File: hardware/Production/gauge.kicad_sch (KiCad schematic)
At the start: 68 parts, among them J105 Cell 2 NTC wires, J106 Cell 3 NTC wires, J108 PACK- power wire, J109 CELL1 sense wire, J110 CELL2 sense wire, J111 CELL3 sense wire, J112 PACK+ power wire, J113 LOAD PACK_P, J114 LOAD GND, J115 1N Kelvin wire, J116 4P Kelvin wire, Q101 BSC007N04LS6, Q102 BSC007N04LS6, Q103 AO3400A, Q104 AO3400A, U101 BQ40Z50RSMR-R2, U102 BQ294700DSGR

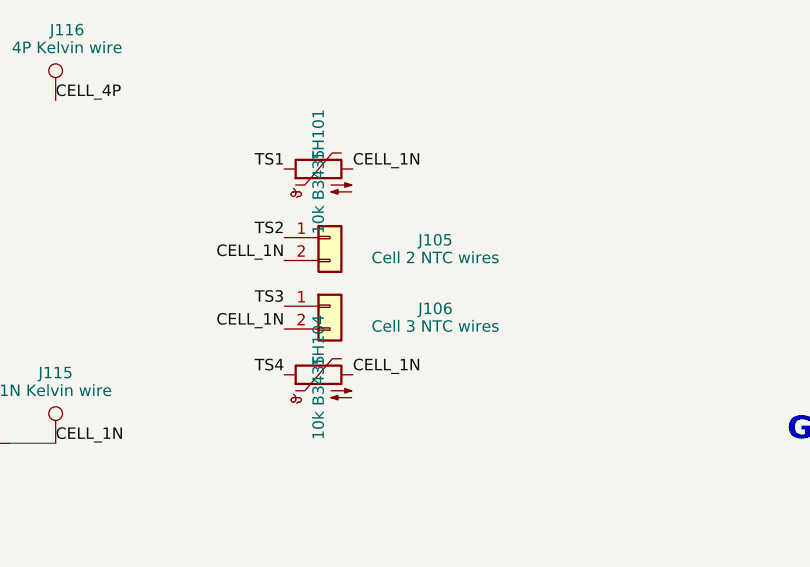
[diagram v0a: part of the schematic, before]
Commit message: Board Layout Done Going to review
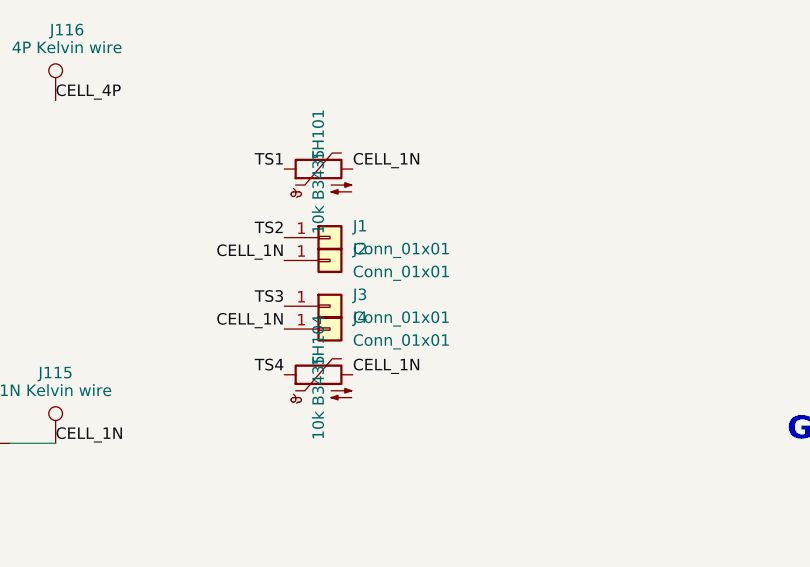
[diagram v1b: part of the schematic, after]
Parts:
- removed J105: Cell 2 NTC wires, Connector_Wire:SolderWire-0.15sqmm_1x02_P4mm_D0.5mm_OD1.5mm, symbol Connector_Generic:Conn_01x02
- removed J106: Cell 3 NTC wires, Connector_Wire:SolderWire-0.15sqmm_1x02_P4mm_D0.5mm_OD1.5mm, symbol Connector_Generic:Conn_01x02
- added J1, J2, J3, J4: Conn_01x01, MonolithDev:SolderWire-28AWG_PTFE_1x01_D0.8mm_Pad1.5x1.4mm, symbol Connector_Generic:Conn_01x01
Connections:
- net CELL_1N: now also J2.1 (Pin_1), J4.1 (Pin_1)
- net TS2: now also J1.1 (Pin_1)
- net TS3: now also J3.1 (Pin_1)

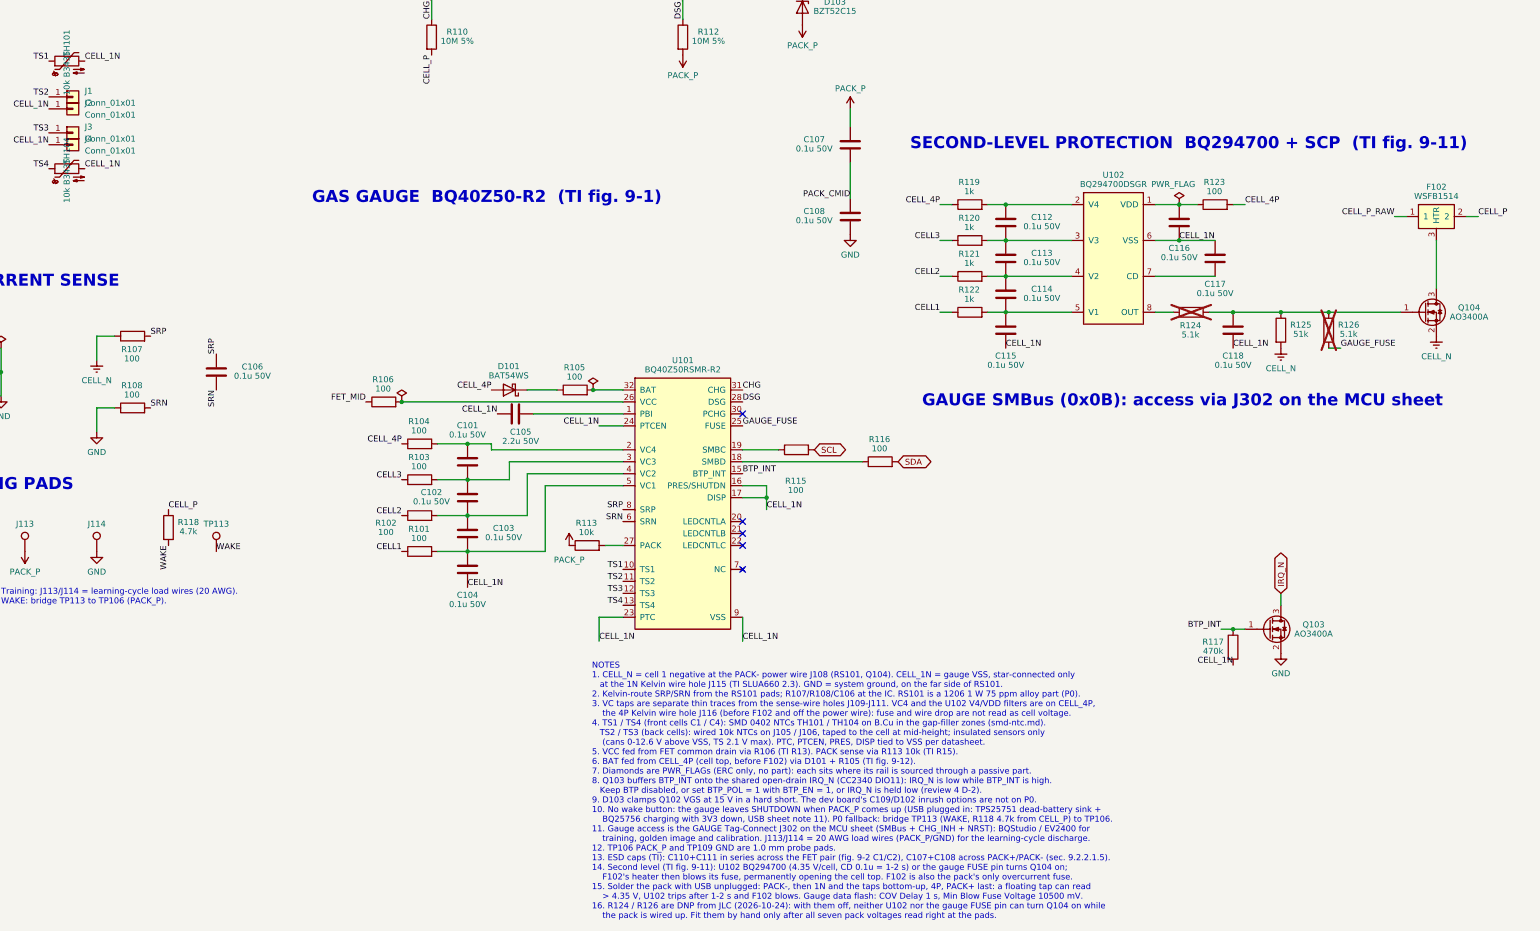
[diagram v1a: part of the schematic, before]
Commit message: Routing fixes done, ready for final review
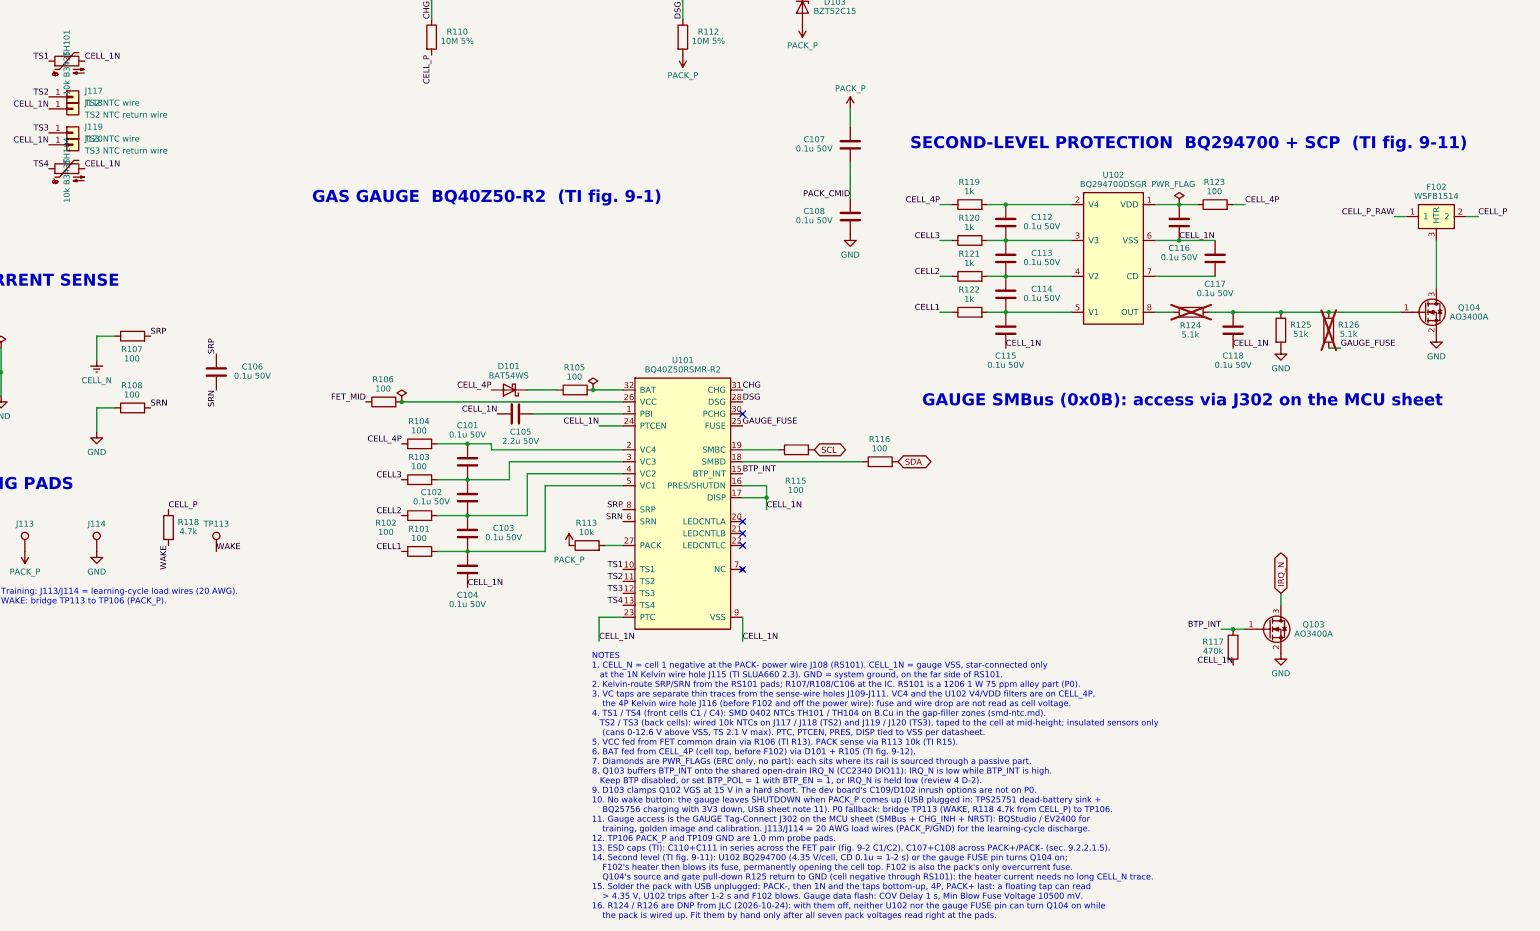
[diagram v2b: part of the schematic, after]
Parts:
- J117: renamed from J1; value Conn_01x01 -> TS2 NTC wire; now left out of the parts list
- J118: renamed from J2; value Conn_01x01 -> TS2 NTC return wire; now left out of the parts list
- J119: renamed from J3; value Conn_01x01 -> TS3 NTC wire; now left out of the parts list
- J120: renamed from J4; value Conn_01x01 -> TS3 NTC return wire; now left out of the parts list
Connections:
- net CELL_N: no longer Q104.2 (S), R125.2
- net GND: now also Q104.2 (S), R125.2
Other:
- note added: "NOTES 1. CELL_N = cell 1 negative at the PACK- power wire J108 (RS101). CELL_1N = gauge VSS, star-connected only at the 1N Kelvin wire hole J115 (TI SLUA660 2.3). GND = system ground, on the far side of RS101. 2. Kelvin-route SRP/SRN from the RS101 pads; R107/R108/C106 at the IC. RS101 is a 1206 1 W 75 ppm alloy part (P0). 3. VC taps are separate thin traces from the sense-wire holes J109-J111. V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"
- note removed: "NOTES 1. CELL_N = cell 1 negative at the PACK- power wire J108 (RS101, Q104). CELL_1N = gauge VSS, star-connected only at the 1N Kelvin wire hole J115 (TI SLUA660 2.3). GND = system ground, on the far side of RS101. 2. Kelvin-route SRP/SRN from the RS101 pads; R107/R108/C106 at the IC. RS101 is a 1206 1 W 75 ppm alloy part (P0). 3. VC taps are separate thin traces from the sense-wire holes J109-J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"
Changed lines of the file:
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@@
 		)
 	)
-	(text "NOTES\n1. CELL_N = cell 1 negative at the PACK- power wire J108 (RS101, Q104). CELL_1N = gauge VSS, star-connected only\n   at the 1N Kelvin wire hole J115 (TI SLUA660 2.3). GND = system ground, on the far side of RS101.\n2. Kelvin-route SRP/SRN from the RS101 pads; R107/R108/C106 at the IC. RS101 is a 1206 1 W 75 ppm alloy part (P0).\n3. VC taps are separate thin traces from the sense-wire holes J109-J111. VC4 and the U102 V4/VDD filters are on CELL_4P,\n    the 4P Kelvin wire hole J116 (before F102 and off the power wire): fuse and wire drop are not read as cell voltage.\n4. TS1 / TS4 (front cells C1 / C4): SMD 0402 NTCs TH101 / TH104 on B.Cu in the gap-filler zones (smd-ntc.md).\n   TS2 / TS3 (back cells): wired 10k NTCs on J105 / J106, taped to the cell at mid-height; insulated sensors only\n    (cans 0-12.6 V above VSS, TS 2.1 V max). PTC, PTCEN, PRES, DISP tied to VSS per datasheet.\n5. VCC fed from FET common drain via R106 (TI R13). PACK sense via R113 10k (TI R15).\n6. BAT fed from CELL_4P (cell top, before F102) via D101 + R105 (TI fig. 9-12).\n7. Diamonds are PWR_FLAGs (ERC only, no part): each sits where its rail is sourced through a passive part.\n8. Q103 buffers BTP_INT onto the shared open-drain IRQ_N (CC2340 DIO11): IRQ_N is low while BTP_INT is high.\n   Keep BTP disabled, or set BTP_POL = 1 with BTP_EN = 1, or IRQ_N is held low (review 4 D-2).\n9. D103 clamps Q102 VGS at 15 V in a hard short. The dev board's C109/D102 inrush options are not on P0.\n10. No wake button: the gauge leaves SHUTDOWN when PACK_P comes up (USB plugged in: TPS25751 dead-battery sink +\n    BQ25756 charging with 3V3 down, USB sheet note 11). P0 fallback: bridge TP113 (WAKE, R118 4.7k from CELL_P) to TP106.\n11. Gauge access is the GAUGE Tag-Connect J302 on the MCU sheet (SMBus + CHG_INH + NRST): BQStudio / EV2400 for\n    training, golden image and calibration. J113/J114 = 20 AWG load wires (PACK_P/GND) for the learning-cycle discharge.\n12. TP106 PACK_P and TP109 GND are 1.0 mm probe pads.\n13. ESD caps (TI): C110+C111 in series across the FET pair (fig. 9-2 C1/C2), C107+C108 across PACK+/PACK- (sec. 9.2.2.1.5).\n14. Second level (TI fig. 9-11): U102 BQ294700 (4.35 V/cell, CD 0.1u = 1-2 s) or the gauge FUSE pin turns Q104 on;\n    F102's heater then blows its fuse, permanently opening the cell top. F102 is also the pack's only overcurrent fuse.\n15. Solder the pack with USB unplugged: PACK-, then 1N and the taps bottom-up, 4P, PACK+ last: a floating tap can read\n    > 4.35 V, U102 trips after 1-2 s and F102 blows. Gauge data flash: COV Delay 1 s, Min Blow Fuse Voltage 10500 mV.\n16. R124 / R126 are DNP from JLC (2026-10-24): with them off, neither U102 nor the gauge FUSE pin can turn Q104 on while\n    the pack is wired up. Fit them by hand only after all seven pack voltages read right at the pads."
+	(text "NOTES\n1. CELL_N = cell 1 negative at the PACK- power wire J108 (RS101). CELL_1N = gauge VSS, star-connected only\n   at the 1N Kelvin wire hole J115 (TI SLUA660 2.3). GND = system ground, on the far side of RS101.\n2. Kelvin-route SRP/SRN from the RS101 pads; R107/R108/C106 at the IC. RS101 is a 1206 1 W 75 ppm alloy part (P0).\n3. VC taps are separate thin traces from the sense-wire holes J109-J111. VC4 and the U102 V4/VDD filters are on CELL_4P,\n    the 4P Kelvin wire hole J116 (before F102 and off the power wire): fuse and wire drop are not read as cell voltage.\n4. TS1 / TS4 (front cells C1 / C4): SMD 0402 NTCs TH101 / TH104 on B.Cu in the gap-filler zones (smd-ntc.md).\n   TS2 / TS3 (back cells): wired 10k NTCs on J117 / J118 (TS2) and J119 / J120 (TS3), taped to the cell at mid-height; insulated sensors only\n    (cans 0-12.6 V above VSS, TS 2.1 V max). PTC, PTCEN, PRES, DISP tied to VSS per datasheet.\n5. VCC fed from FET common drain via R106 (TI R13). PACK sense via R113 10k (TI R15).\n6. BAT fed from CELL_4P (cell top, before F102) via D101 + R105 (TI fig. 9-12).\n7. Diamonds are PWR_FLAGs (ERC only, no part): each sits where its rail is sourced through a passive part.\n8. Q103 buffers BTP_INT onto the shared open-drain IRQ_N (CC2340 DIO11): IRQ_N is low while BTP_INT is high.\n   Keep BTP disabled, or set BTP_POL = 1 with BTP_EN = 1, or IRQ_N is held low (review 4 D-2).\n9. D103 clamps Q102 VGS at 15 V in a hard short. The dev board's C109/D102 inrush options are not on P0.\n10. No wake button: the gauge leaves SHUTDOWN when PACK_P comes up (USB plugged in: TPS25751 dead-battery sink +\n    BQ25756 charging with 3V3 down, USB sheet note 11). P0 fallback: bridge TP113 (WAKE, R118 4.7k from CELL_P) to TP106.\n11. Gauge access is the GAUGE Tag-Connect J302 on the MCU sheet (SMBus + CHG_INH + NRST): BQStudio / EV2400 for\n    training, golden image and calibration. J113/J114 = 20 AWG load wires (PACK_P/GND) for the learning-cycle discharge.\n12. TP106 PACK_P and TP109 GND are 1.0 mm probe pads.\n13. ESD caps (TI): C110+C111 in series across the FET pair (fig. 9-2 C1/C2), C107+C108 across PACK+/PACK- (sec. 9.2.2.1.5).\n14. Second level (TI fig. 9-11): U102 BQ294700 (4.35 V/cell, CD 0.1u = 1-2 s) or the gauge FUSE pin turns Q104 on;\n    F102's heater then blows its fuse, permanently opening the cell top. F102 is also the pack's only overcurrent fuse.\n    Q104's source and gate pull-down R125 return to GND (cell negative through RS101): the heater current needs no long CELL_N trace.\n15. Solder the pack with USB unplugged: PACK-, then 1N and the taps bottom-up, 4P, PACK+ last: a floating tap can read\n    > 4.35 V, U102 trips after 1-2 s and F102 blows. Gauge data flash: COV Delay 1 s, Min Blow Fuse Voltage 10500 mV.\n16. R124 / R126 are DNP from JLC (2026-10-24): with them off, neither U102 nor the gauge FUSE pin can turn Q104 on while\n    the pack is wired up. Fit them by hand only after all seven pack voltages read right at the pads."
 		(exclude_from_sim no)
 		(at 196.596 248.412 0)
@@
 		(body_style 1)
 		(exclude_from_sim no)
-		(in_bom yes)
+		(in_bom no)
 		(on_board yes)
 		(in_pos_files yes)
 		(dnp no)
 		(fields_autoplaced yes)
-		(property "Reference" "J1"
+		(property "Reference" "J117"
 			(at 88.9 72.3899 0)
 			(show_name no)
@@
 			)
 		)
-		(property "Value" "Conn_01x01"
+		(property "Value" "TS2 NTC wire"
 			(at 88.9 74.9299 0)
 			(show_name no)
@@
 			(project "Monolith"
 				(path "/f83241ae-2bb3-4ed7-b986-c0a03971de0a/5f8e2264-136e-4c01-877f-88ca3aa05650"
-					(reference "J1")
+					(reference "J117")
 					(unit 1)
 				)
@@
 		(body_style 1)
 		(exclude_from_sim no)
-		(in_bom yes)
+		(in_bom no)
 		(on_board yes)
 		(in_pos_files yes)
 		(dnp no)
 		(fields_autoplaced yes)
-		(property "Reference" "J3"
+		(property "Reference" "J119"
 			(at 88.9 80.0099 0)
 			(show_name no)
@@
 			)
 		)
-		(property "Value" "Conn_01x01"
+		(property "Value" "TS3 NTC wire"
 			(at 88.9 82.5499 0)
 			(show_name no)
@@
 			(project "Monolith"
 				(path "/f83241ae-2bb3-4ed7-b986-c0a03971de0a/5f8e2264-136e-4c01-877f-88ca3aa05650"
-					(reference "J3")
+					(reference "J119")
 					(unit 1)
 				)
@@
 	)
 	(symbol
-		(lib_id "power:GNDREF")
+		(lib_id "power:GND")
 		(at 375.92 124.46 0)
 		(unit 1)
@@
 			)
 		)
-		(property "Value" "CELL_N"
+		(property "Value" "GND"
 			(at 375.92 128.78 0)
 			(show_name no)
@@
 		(body_style 1)
 		(exclude_from_sim no)
-		(in_bom yes)
+		(in_bom no)
 		(on_board yes)
 		(in_pos_files yes)
 		(dnp no)
 		(fields_autoplaced yes)
-		(property "Reference" "J2"
+		(property "Reference" "J118"
 			(at 88.9 74.9299 0)
 			(show_name no)
@@
 			)
 		)
-		(property "Value" "Conn_01x01"
+		(property "Value" "TS2 NTC return wire"
 			(at 88.9 77.4699 0)
 			(show_name no)
@@
 			(project "Monolith"
 				(path "/f83241ae-2bb3-4ed7-b986-c0a03971de0a/5f8e2264-136e-4c01-877f-88ca3aa05650"
-					(reference "J2")
+					(reference "J118")
 					(unit 1)
 				)
@@
 		(body_style 1)
 		(exclude_from_sim no)
-		(in_bom yes)
+		(in_bom no)
 		(on_board yes)
 		(in_pos_files yes)
 		(dnp no)
 		(fields_autoplaced yes)
-		(property "Reference" "J4"
+		(property "Reference" "J120"
 			(at 88.9 82.5499 0)
 			(show_name no)
@@
 			)
 		)
-		(property "Value" "Conn_01x01"
+		(property "Value" "TS3 NTC return wire"
 			(at 88.9 85.0899 0)
 			(show_name no)
@@
 			(project "Monolith"
 				(path "/f83241ae-2bb3-4ed7-b986-c0a03971de0a/5f8e2264-136e-4c01-877f-88ca3aa05650"
-					(reference "J4")
+					(reference "J120")
 					(unit 1)
 				)
@@
 	)
 	(symbol
-		(lib_id "power:GNDREF")
+		(lib_id "power:GND")
 		(at 342.9 127 0)
 		(unit 1)
@@
 			)
 		)
-		(property "Value" "CELL_N"
+		(property "Value" "GND"
 			(at 342.9 131.32 0)
 			(show_name no)
